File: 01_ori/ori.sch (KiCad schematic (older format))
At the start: 131 parts, among them J1 TYPE-C-31-M12_13, J2 AVR-ISP-6_mod, K1 KEYSW, K10 KEYSW, K11 KEYSW, K12 KEYSW, K13 KEYSW, K14 KEYSW, K15 KEYSW, K16 KEYSW, K17 KEYSW, K18 KEYSW, K19 KEYSW, K2 KEYSW, K20 KEYSW, K21 KEYSW, K22 KEYSW, K23 KEYSW, K24 KEYSW, K25 KEYSW, K26 KEYSW, K27 KEYSW, K28 KEYSW, K29 KEYSW, K3 KEYSW, K30 KEYSW, K31 KEYSW, K32 KEYSW, K33 KEYSW, K34 KEYSW, K35 KEYSW, K36 KEYSW, K37 KEYSW, K38 KEYSW, K39 KEYSW, K4 KEYSW, K40 KEYSW, K41 KEYSW, K42 KEYSW, K43 KEYSW, K44 KEYSW, K45 KEYSW, K46 KEYSW, K47 KEYSW, K48 KEYSW, K49 KEYSW, K5 KEYSW, K50 KEYSW, K51 KEYSW, K52 KEYSW, K6 KEYSW, K7 KEYSW, K8 KEYSW, K9 KEYSW, SW1 SW_PUSH, SW2 Rotary_Encoder_Switch, U1 ATMEGA32U4, Y1 16MHz

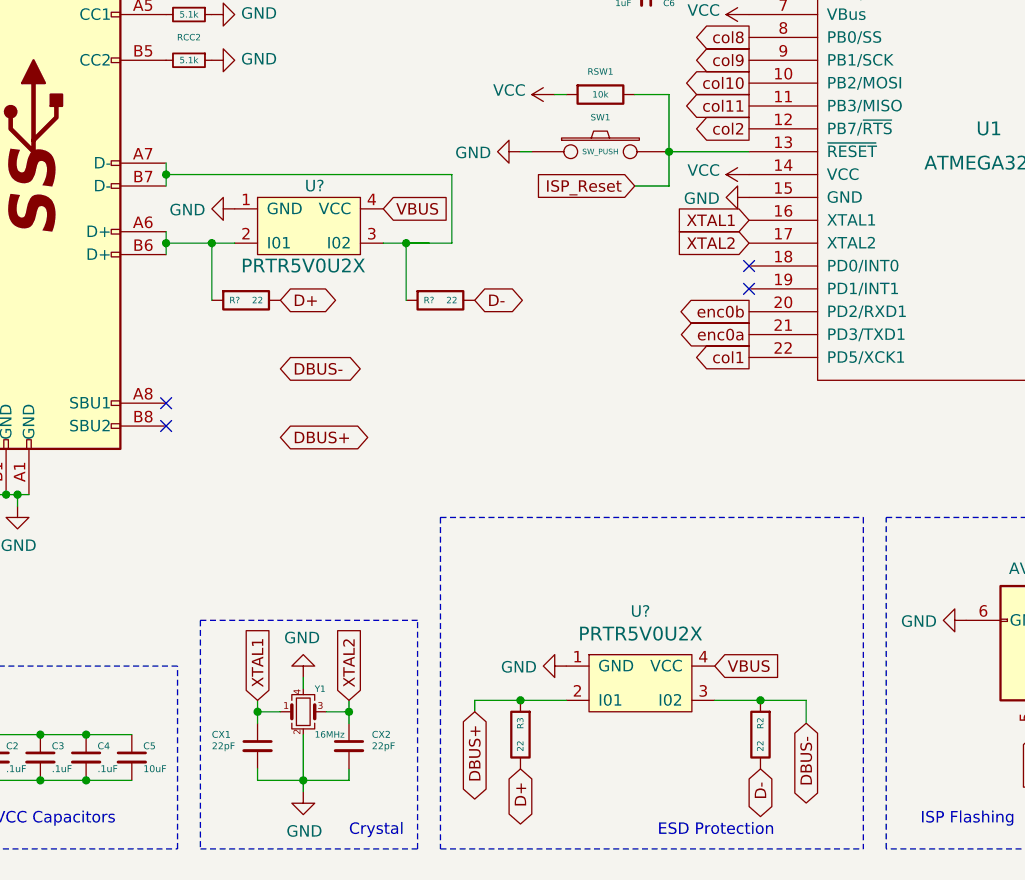
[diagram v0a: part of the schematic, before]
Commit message: update rev silkscreen
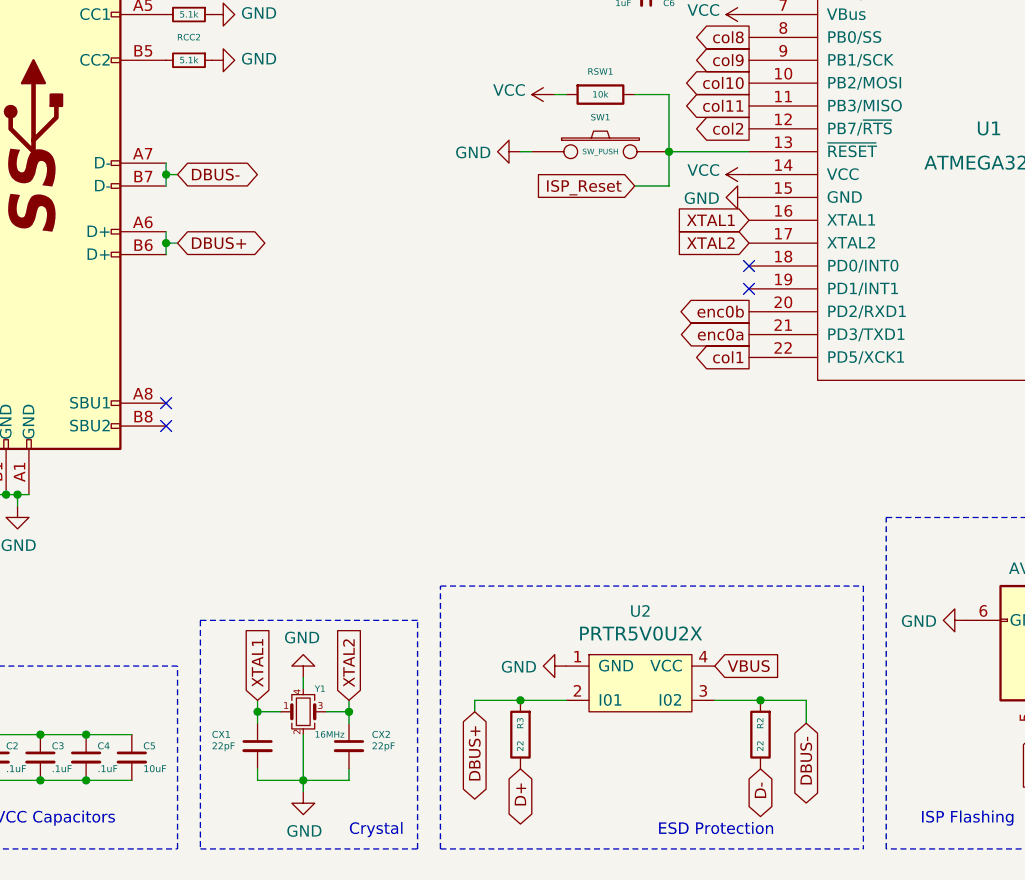
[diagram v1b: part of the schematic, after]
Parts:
- removed R? (x2): 22, Resistor_SMD:R_0805_2012Metric_Pad1.15x1.40mm_HandSolder, symbol Device:R
- removed U?: PRTR5V0U2X, symbol keyboard_parts:PRTR5V0U2X
- U2: renamed from U?; footprint (none) -> Keebio-Parts:SOT-143B
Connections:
- net DBUS+: now also J1.A6 (D+), J1.B6 (D+)
- net DBUS-: now also J1.A7 (D-), J1.B7 (D-)
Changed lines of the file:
@@
 Text GLabel 5300 6900 0    50   Input ~ 0
 XTAL2
-Text GLabel 3250 7750 2    50   BiDi ~ 0
-DBUS+
-Text GLabel 3250 7450 2    50   BiDi ~ 0
-DBUS-
 Text GLabel 7450 6000 2    50   Output ~ 0
 row1
@@
 	0    1    1    0
 $EndComp
-Wire Notes Line
-	3950 8100 3950 9550
 Text GLabel 4800 6650 0    50   Input ~ 0
 ISP_Reset
@@
 $EndComp
 Wire Notes Line
-	5800 8100 5800 9550
-Wire Notes Line
-	3950 8100 5800 8100
-Wire Notes Line
 	3950 9550 5800 9550
 $Comp
@@
 DBUS+
 $Comp
-L keyboard_parts:PRTR5V0U2X U?
+L keyboard_parts:PRTR5V0U2X U2
 U 1 1 616D1410
 P 4800 8600
-F 0 "U?" H 4825 8689 50  0000 C CNN
+F 0 "U2" H 4825 8689 50  0000 C CNN
 F 1 "PRTR5V0U2X" H 4825 8590 60  0000 C CNN
-F 2 "" H 4800 8600 50  0001 C CNN
+F 2 "Keebio-Parts:SOT-143B" H 4800 8600 50  0001 C CNN
 F 3 "" H 4800 8600 50  0001 C CNN
 	1    4800 8600
 	1    0    0    -1
 $EndComp
-Text GLabel 3250 7150 2    50   BiDi ~ 0
-D+
 $Comp
 L Device:R R3
@@
 Text Notes 4900 9500 0    50   ~ 0
 ESD Protection
-$Comp
-L keyboard_parts:PRTR5V0U2X U?
-U 1 1 61869AB0
-P 3350 6600
-F 0 "U?" H 3400 6550 50  0000 C CNN
-F 1 "PRTR5V0U2X" H 3350 6200 60  0000 C CNN
-F 2 "" H 3350 6600 50  0001 C CNN
-F 3 "" H 3350 6600 50  0001 C CNN
-	1    3350 6600
-	1    0    0    -1
-$EndComp
-Wire Wire Line
-	3050 6900 2950 6900
-Connection ~ 2950 6900
-Wire Wire Line
-	2950 6900 2950 7150
-Wire Wire Line
-	2750 6550 2750 6600
-Wire Wire Line
-	2750 6850 2750 6900
-Wire Wire Line
-	2750 6900 2950 6900
-Connection ~ 2750 6900
-Wire Wire Line
-	2750 6900 2750 6950
-Connection ~ 2750 6600
-Wire Wire Line
-	2750 6600 2750 6650
-Wire Wire Line
-	3800 6900 3800 7150
-Connection ~ 3800 6900
-Wire Wire Line
-	3800 6900 3700 6900
 Wire Wire Line
 	4500 8900 4300 8900
@@
 Text GLabel 4300 9200 3    50   BiDi ~ 0
 D+
-$Comp
-L Device:R R?
-U 1 1 61AB31D0
-P 3100 7150
-F 0 "R?" V 3100 7100 28  0000 C CNN
-F 1 "22" V 3100 7200 28  0000 C CNN
-F 2 "Resistor_SMD:R_0805_2012Metric_Pad1.15x1.40mm_HandSolder" V 3030 7150 50  0001 C CNN
-F 3 "~" H 3100 7150 50  0001 C CNN
-	1    3100 7150
-	0    1    1    0
-$EndComp
 Wire Wire Line
 	5150 8900 5350 8900
@@
 	-1   0    0    1
 $EndComp
-Text GLabel 4100 7150 2    50   BiDi ~ 0
-D-
-$Comp
-L Device:R R?
-U 1 1 61B0952A
-P 3950 7150
-F 0 "R?" V 3950 7100 28  0000 C CNN
-F 1 "22" V 3950 7200 28  0000 C CNN
-F 2 "Resistor_SMD:R_0805_2012Metric_Pad1.15x1.40mm_HandSolder" V 3880 7150 50  0001 C CNN
-F 3 "~" H 3950 7150 50  0001 C CNN
-	1    3950 7150
-	0    1    1    0
-$EndComp
 Text GLabel 5350 9200 3    50   BiDi ~ 0
 D-
-$Comp
-L power:GND #PWR?
-U 1 1 61B33909
-P 3050 6750
-F 0 "#PWR?" H 3050 6500 50  0001 C CNN
-F 1 "GND" V 3055 6622 50  0000 R CNN
-F 2 "" H 3050 6750 50  0001 C CNN
-F 3 "" H 3050 6750 50  0001 C CNN
-	1    3050 6750
-	0    1    1    0
-$EndComp
-Text GLabel 3700 6750 2    50   Input ~ 0
-VBUS
-Wire Wire Line
-	4000 6600 4000 6900
-Wire Wire Line
-	3900 6900 3800 6900
-Wire Wire Line
-	2750 6600 4000 6600
-Wire Wire Line
-	3800 6900 4000 6900
 $Comp
 L Ori-rescue:TYPE-C-31-M12_13-acheronSymbols J1
@@
 Wire Wire Line
 	5350 8900 5550 8900
+Text GLabel 2800 6600 2    50   BiDi ~ 0
+DBUS-
+Text GLabel 2800 6900 2    50   BiDi ~ 0
+DBUS+
+Wire Wire Line
+	2750 6550 2750 6600
+Wire Wire Line
+	2750 6850 2750 6900
+Wire Wire Line
+	2800 6600 2750 6600
+Connection ~ 2750 6600
+Wire Wire Line
+	2750 6600 2750 6650
+Wire Wire Line
+	2800 6900 2750 6900
+Connection ~ 2750 6900
+Wire Wire Line
+	2750 6900 2750 6950
+Wire Notes Line
+	3950 9550 3950 8400
+Wire Notes Line
+	3950 8400 5800 8400
+Wire Notes Line
+	5800 8400 5800 9550
 $EndSCHEMATC
